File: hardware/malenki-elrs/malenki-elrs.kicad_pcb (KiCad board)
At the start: 4 copper layers, 19 x 32 mm, 62 parts, among them J1 Conn_01x02_Male-Connector, J2 PROG Header, J3 Weapons, J4 Conn_01x02_Male-Connector, J5 Conn_01x02_Male-Connector, J6 Conn_01x02_Male-Connector, U1 SPX3819M5-L-3-3, U3 SX1280IMLTRT, U4 DRV8837DSGR, U5 DRV8837DSGR, U6 DRV8837DSGR, U7 ESP32-S3FN8, Y1 ECS-400-10-37B2-CKY-TR, Y2 CRYSTAL 52MHz 10pF SMD

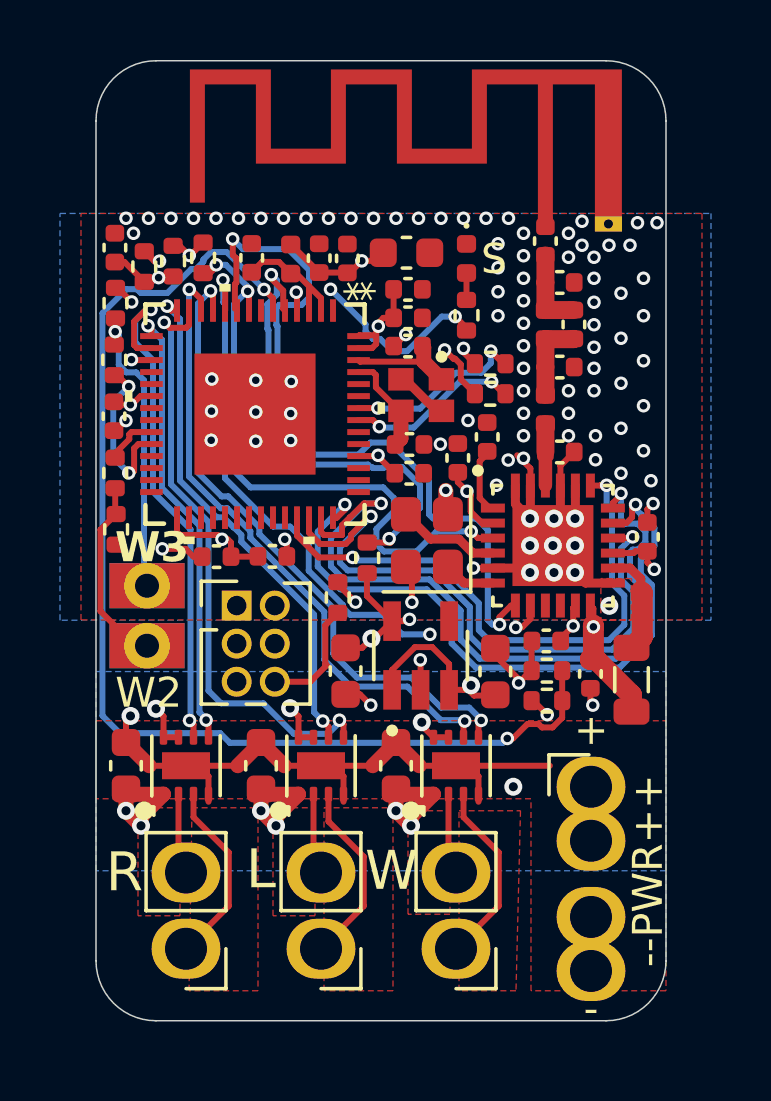
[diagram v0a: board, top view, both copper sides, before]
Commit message: Generated production files
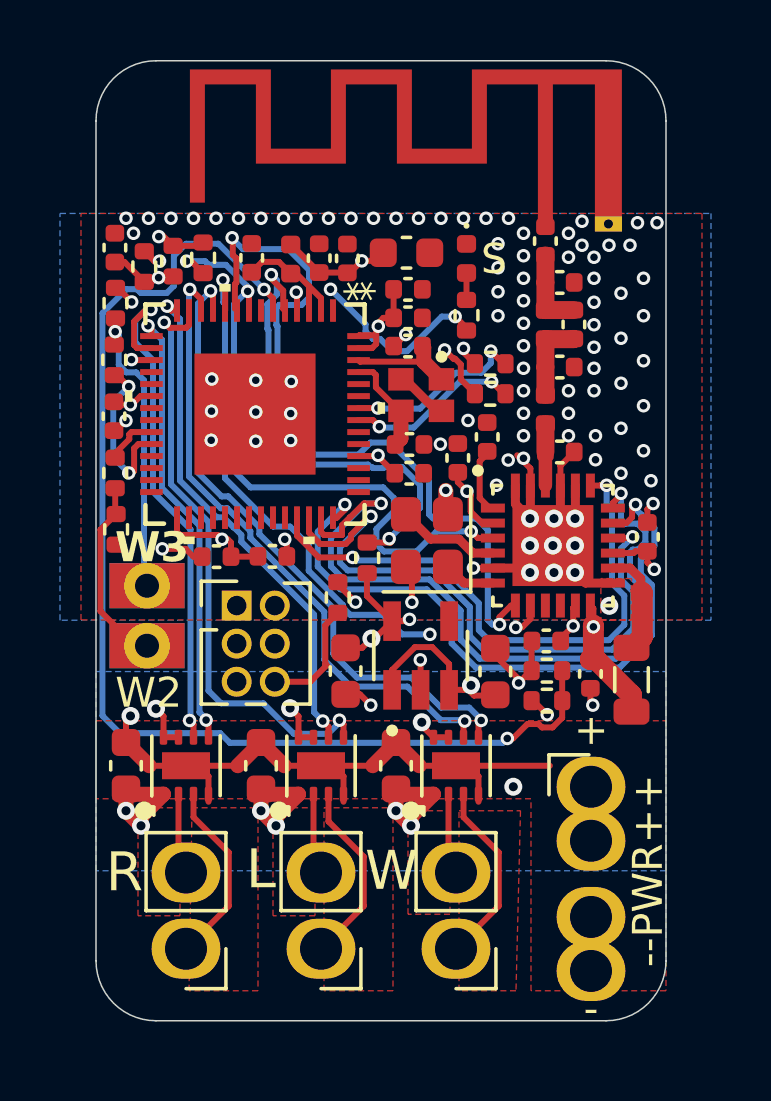
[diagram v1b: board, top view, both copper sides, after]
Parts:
- renumbered U7 to U2
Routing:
- net RADIO_NRESET: track 20.8 -> 21.9 mm
- net VSENSE: track 38.8 -> 39.6 mm
